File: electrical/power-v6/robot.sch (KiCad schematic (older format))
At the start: 24 parts, among them J1 C1-2, J10 LEG2, J11 EXT, J12 LEG4, J13 EXT, J14 C3-4, J15 LEG3, J16 5V, J17 12V, J18 12V, J2 RPi, J3 Data, J4 Leg1-2, J5 USB_A, J6 5V Pwr, J7 Leg3-4, J8 LEG1, J9 5V

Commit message: new board :electric_plug:  :bento:
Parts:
- D1: symbol Device:LED -> robot-rescue:LED-Device
- H1, H2, H3, H4: symbol Mechanical:MountingHole -> robot-rescue:MountingHole-Mechanical
- J16, J17, J18, J9: symbol Connector_Generic:Conn_01x02 -> robot-rescue:Conn_01x02-Connector_Generic
- J4, J7: footprint Wire_Connections_Bridges:WireConnection_2.50mmDrill_LargePad -> Wire_Connections_Bridges:WireConnection_1.50mmDrill; symbol Connector_Generic:Conn_01x02 -> robot-rescue:Conn_01x02-Connector_Generic
- J5: symbol Connector:USB_A -> robot-rescue:USB_A-Connector
- J6: symbol Connector_Generic:Conn_01x05 -> robot-rescue:Conn_01x05-Connector_Generic
- R1: symbol Device:R -> robot-rescue:R-Device
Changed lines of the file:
@@
 $EndComp
 $Comp
-L power:PWR_FLAG #FLG01
+L robot-rescue:PWR_FLAG-power #FLG01
 U 1 1 5A7F9C06
 P 2150 7050
@@
 $EndComp
 $Comp
-L power:PWR_FLAG #FLG02
+L robot-rescue:PWR_FLAG-power #FLG02
 U 1 1 5A935890
 P 1500 7150
@@
 $EndComp
 $Comp
-L power:+12V #PWR03
+L robot-rescue:+12V-power #PWR03
 U 1 1 5AA56F03
 P 1500 7050
@@
 $EndComp
 $Comp
-L power:GND #PWR04
+L robot-rescue:GND-power #PWR04
 U 1 1 5AA58E71
 P 2150 7150
@@
 $EndComp
 $Comp
-L Device:LED D1
+L robot-rescue:LED-Device D1
 U 1 1 5ACD24C2
 P 5850 2850
@@
 $EndComp
 $Comp
-L Device:R R1
+L robot-rescue:R-Device R1
 U 1 1 5ACD2583
 P 5850 3300
@@
 $EndComp
 $Comp
-L power:GND #PWR06
+L robot-rescue:GND-power #PWR06
 U 1 1 5ACD2691
 P 5850 3600
@@
 $EndComp
 $Comp
-L power:GND #PWR07
+L robot-rescue:GND-power #PWR07
 U 1 1 5ACD2D22
 P 6850 5700
@@
 $EndComp
 $Comp
-L power:GND #PWR08
+L robot-rescue:GND-power #PWR08
 U 1 1 5ACD2DD3
 P 9000 5700
@@
 	6650 2400 6600 2400
 $Comp
-L Connector:USB_A J5
+L robot-rescue:USB_A-Connector J5
 U 1 1 5BF9F178
 P 5400 4250
@@
 $EndComp
 $Comp
-L Connector_Generic:Conn_01x05 J6
+L robot-rescue:Conn_01x05-Connector_Generic J6
 U 1 1 5BFA49E0
 P 6200 4900
@@
 NoConn ~ 6400 5100
 $Comp
-L power:GND #PWR0101
+L robot-rescue:GND-power #PWR0101
 U 1 1 5BFB9CA6
 P 5400 4800
@@
 NoConn ~ 5700 4350
 $Comp
-L power:+5V #PWR0102
+L robot-rescue:+5V-power #PWR0102
 U 1 1 5BFC6D63
 P 5850 4050
@@
 $EndComp
 $Comp
-L power:+5V #PWR0103
+L robot-rescue:+5V-power #PWR0103
 U 1 1 5BFC6E0E
 P 6950 4600
@@
 $EndComp
 $Comp
-L power:+5V #PWR0104
+L robot-rescue:+5V-power #PWR0104
 U 1 1 5BFC6E39
 P 6500 4600
@@
 	6950 4700 6950 4600
 $Comp
-L power:+5V #PWR0105
+L robot-rescue:+5V-power #PWR0105
 U 1 1 5BFCCF39
 P 1000 7050
@@
 $EndComp
 $Comp
-L power:PWR_FLAG #FLG0101
+L robot-rescue:PWR_FLAG-power #FLG0101
 U 1 1 5BFCD434
 P 1000 7150
@@
 Connection ~ 6950 4100
 $Comp
-L Mechanical:MountingHole H1
+L robot-rescue:MountingHole-Mechanical H1
 U 1 1 5BFD2444
 P 8950 700
@@
 $EndComp
 $Comp
-L Mechanical:MountingHole H2
+L robot-rescue:MountingHole-Mechanical H2
 U 1 1 5BFD296E
 P 8950 900
@@
 $EndComp
 $Comp
-L Mechanical:MountingHole H3
+L robot-rescue:MountingHole-Mechanical H3
 U 1 1 5BFD29A2
 P 8950 1100
@@
 $EndComp
 $Comp
-L Mechanical:MountingHole H4
+L robot-rescue:MountingHole-Mechanical H4
 U 1 1 5BFD29D8
 P 8950 1300
@@
 $EndComp
 $Comp
-L Connector_Generic:Conn_01x02 J4
+L robot-rescue:Conn_01x02-Connector_Generic J4
 U 1 1 5BFB1889
 P 6400 2500
 F 0 "J4" H 6320 2175 50  0000 C CNN
 F 1 "Leg1-2" H 6320 2266 50  0000 C CNN
-F 2 "Wire_Connections_Bridges:WireConnection_2.50mmDrill_LargePad" H 6400 2500 50  0001 C CNN
+F 2 "Wire_Connections_Bridges:WireConnection_1.50mmDrill" H 6400 2500 50  0001 C CNN
 F 3 "~" H 6400 2500 50  0001 C CNN
 	1    6400 2500
@@
 $EndComp
 $Comp
-L Connector_Generic:Conn_01x02 J7
+L robot-rescue:Conn_01x02-Connector_Generic J7
 U 1 1 5BFB1BE8
 P 8550 2500
 F 0 "J7" H 8470 2175 50  0000 C CNN
 F 1 "Leg3-4" H 8470 2266 50  0000 C CNN
-F 2 "Wire_Connections_Bridges:WireConnection_2.50mmDrill_LargePad" H 8550 2500 50  0001 C CNN
+F 2 "Wire_Connections_Bridges:WireConnection_1.50mmDrill" H 8550 2500 50  0001 C CNN
 F 3 "~" H 8550 2500 50  0001 C CNN
 	1    8550 2500
@@
 $EndComp
 $Comp
-L Connector_Generic:Conn_01x02 J17
+L robot-rescue:Conn_01x02-Connector_Generic J17
 U 1 1 5BFBD4E7
 P 9550 5000
@@
 $EndComp
 $Comp
-L Connector_Generic:Conn_01x02 J18
+L robot-rescue:Conn_01x02-Connector_Generic J18
 U 1 1 5BFBD5C7
 P 9550 5300
@@
 $EndComp
 $Comp
-L Connector_Generic:Conn_01x02 J9
+L robot-rescue:Conn_01x02-Connector_Generic J9
 U 1 1 5BFBD605
 P 7400 5050
@@
 $EndComp
 $Comp
-L Connector_Generic:Conn_01x02 J16
+L robot-rescue:Conn_01x02-Connector_Generic J16
 U 1 1 5BFBD645
 P 7400 5350

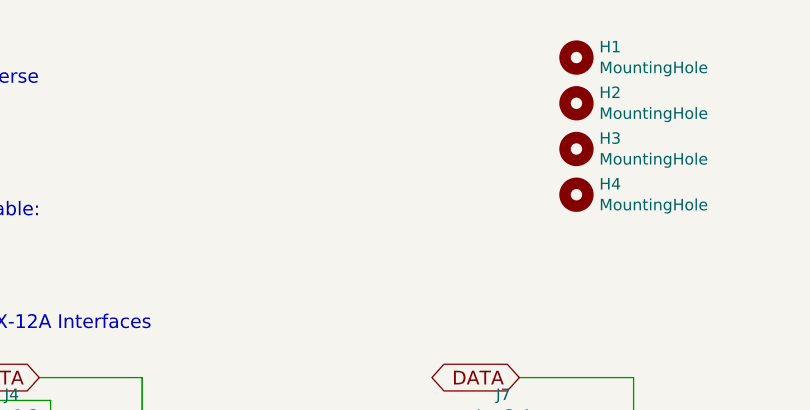
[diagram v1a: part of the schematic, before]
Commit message: up
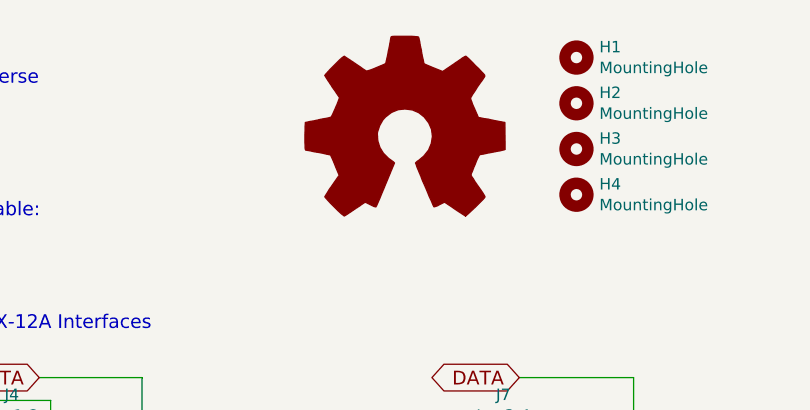
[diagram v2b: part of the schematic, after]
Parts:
- added LOGO1: Logo_Open_Hardware_Large, Symbol:OSHW-Logo2_24.3x20mm_SilkScreen, symbol Graphic:Logo_Open_Hardware_Large
- H1, H2, H3, H4: footprint Mounting_Holes:MountingHole_2.2mm_M2 -> MountingHole:MountingHole_2.5mm
- J5: footprint Connectors:USB_A -> Connector_USB:USB_A_Wuerth_61400826021_Horizontal_Stacked
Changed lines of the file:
@@
 F 0 "J5" H 5455 4717 50  0000 C CNN
 F 1 "USB_A" H 5455 4626 50  0000 C CNN
-F 2 "Connectors:USB_A" H 5550 4200 50  0001 C CNN
+F 2 "Connector_USB:USB_A_Wuerth_61400826021_Horizontal_Stacked" H 5550 4200 50  0001 C CNN
 F 3 " ~" H 5550 4200 50  0001 C CNN
 	1    5400 4250
@@
 F 0 "H1" H 9050 746 50  0000 L CNN
 F 1 "MountingHole" H 9050 655 50  0000 L CNN
-F 2 "Mounting_Holes:MountingHole_2.2mm_M2" H 8950 700 50  0001 C CNN
+F 2 "MountingHole:MountingHole_2.5mm" H 8950 700 50  0001 C CNN
 F 3 "~" H 8950 700 50  0001 C CNN
 	1    8950 700
@@
 F 0 "H2" H 9050 946 50  0000 L CNN
 F 1 "MountingHole" H 9050 855 50  0000 L CNN
-F 2 "Mounting_Holes:MountingHole_2.2mm_M2" H 8950 900 50  0001 C CNN
+F 2 "MountingHole:MountingHole_2.5mm" H 8950 900 50  0001 C CNN
 F 3 "~" H 8950 900 50  0001 C CNN
 	1    8950 900
@@
 F 0 "H3" H 9050 1146 50  0000 L CNN
 F 1 "MountingHole" H 9050 1055 50  0000 L CNN
-F 2 "Mounting_Holes:MountingHole_2.2mm_M2" H 8950 1100 50  0001 C CNN
+F 2 "MountingHole:MountingHole_2.5mm" H 8950 1100 50  0001 C CNN
 F 3 "~" H 8950 1100 50  0001 C CNN
 	1    8950 1100
@@
 F 0 "H4" H 9050 1346 50  0000 L CNN
 F 1 "MountingHole" H 9050 1255 50  0000 L CNN
-F 2 "Mounting_Holes:MountingHole_2.2mm_M2" H 8950 1300 50  0001 C CNN
+F 2 "MountingHole:MountingHole_2.5mm" H 8950 1300 50  0001 C CNN
 F 3 "~" H 8950 1300 50  0001 C CNN
 	1    8950 1300
@@
 Wire Wire Line
 	9000 5400 9000 5700
+$Comp
+L Graphic:Logo_Open_Hardware_Large LOGO1
+U 1 1 5BFF3E95
+P 8200 1050
+F 0 "LOGO1" H 8200 1550 50  0001 C CNN
+F 1 "Logo_Open_Hardware_Large" H 8200 650 50  0001 C CNN
+F 2 "Symbol:OSHW-Logo2_24.3x20mm_SilkScreen" H 8200 1050 50  0001 C CNN
+F 3 "~" H 8200 1050 50  0001 C CNN
+	1    8200 1050
+	1    0    0    -1
+$EndComp
 $EndSCHEMATC
